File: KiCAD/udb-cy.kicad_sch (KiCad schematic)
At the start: 15 parts, among them J0 USB_C_Receptacle, J1 JST-SH-04, J2 JST-SUR-04, J3 Conn_01x04

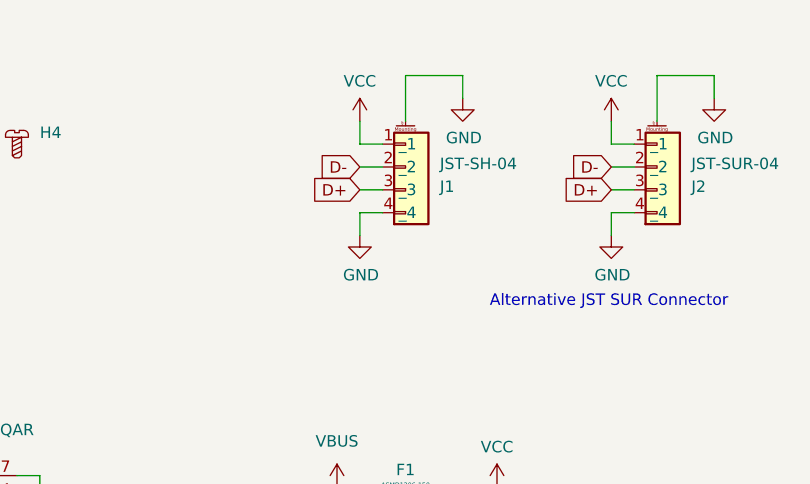
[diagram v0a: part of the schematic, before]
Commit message: update-2025-11-20
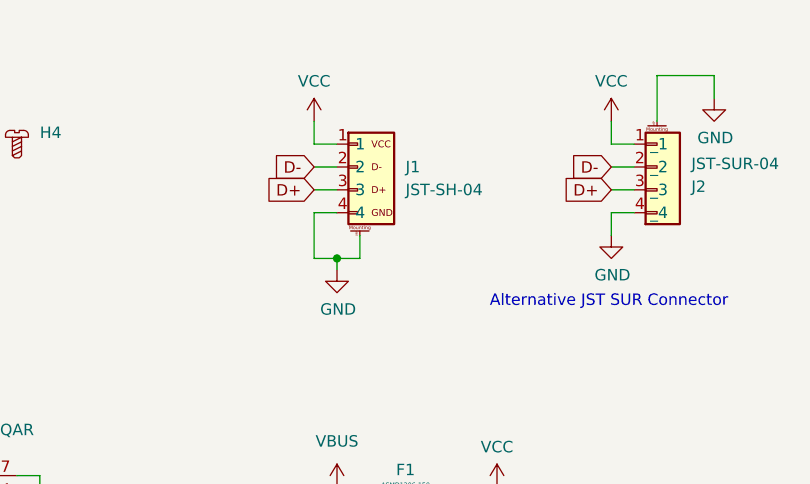
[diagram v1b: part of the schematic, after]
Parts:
- J1: symbol ts-kicad-lib:CONN_04 -> ts-keyboard-lib:CONN_UDB
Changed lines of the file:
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@@
+	)
+	(junction
+		(at 144.78 48.26)
+		(diameter 0)
+		(color 0 0 0 0)
 	)
 	(junction
@@
 	(wire
 		(pts
-			(xy 147.32 45.72) (xy 147.32 43.18)
+			(xy 144.78 49.53) (xy 144.78 48.26)
 		)
 		(stroke
@@
 	(wire
 		(pts
-			(xy 152.4 27.94) (xy 152.4 33.02)
-		)
-		(stroke
-			(width 0)
-			(type default)
-		)
-	)
-	(wire
-		(pts
 			(xy 38.1 78.74) (xy 38.1 83.82)
 		)
@@
 	(wire
 		(pts
+			(xy 144.78 48.26) (xy 142.24 48.26)
+		)
+		(stroke
+			(width 0)
+			(type default)
+		)
+	)
+	(wire
+		(pts
 			(xy 144.78 76.2) (xy 148.59 76.2)
 		)
@@
 	(wire
 		(pts
-			(xy 147.32 40.64) (xy 149.86 40.64)
-		)
-		(stroke
-			(width 0)
-			(type default)
-		)
-	)
-	(wire
-		(pts
 			(xy 156.21 76.2) (xy 160.02 76.2)
 		)
@@
 	(wire
 		(pts
+			(xy 147.32 45.72) (xy 147.32 48.26)
+		)
+		(stroke
+			(width 0)
+			(type default)
+		)
+	)
+	(wire
+		(pts
 			(xy 45.72 43.18) (xy 50.8 43.18)
 		)
@@
 	(wire
 		(pts
+			(xy 142.24 43.18) (xy 144.78 43.18)
+		)
+		(stroke
+			(width 0)
+			(type default)
+		)
+	)
+	(wire
+		(pts
 			(xy 180.34 27.94) (xy 180.34 33.02)
 		)
@@
 	(wire
 		(pts
+			(xy 144.78 48.26) (xy 147.32 48.26)
+		)
+		(stroke
+			(width 0)
+			(type default)
+		)
+	)
+	(wire
+		(pts
 			(xy 66.04 45.72) (xy 50.8 45.72)
 		)
@@
 	(wire
 		(pts
-			(xy 158.75 27.94) (xy 152.4 27.94)
-		)
-		(stroke
-			(width 0)
-			(type default)
-		)
-	)
-	(wire
-		(pts
-			(xy 147.32 33.02) (xy 147.32 35.56)
+			(xy 142.24 33.02) (xy 142.24 35.56)
 		)
 		(stroke
@@
 	(wire
 		(pts
+			(xy 142.24 38.1) (xy 144.78 38.1)
+		)
+		(stroke
+			(width 0)
+			(type default)
+		)
+	)
+	(wire
+		(pts
 			(xy 48.26 86.36) (xy 50.8 86.36)
 		)
@@
 	(wire
 		(pts
+			(xy 142.24 48.26) (xy 142.24 43.18)
+		)
+		(stroke
+			(width 0)
+			(type default)
+		)
+	)
+	(wire
+		(pts
 			(xy 109.22 80.01) (xy 111.76 80.01)
 		)
@@
 	(wire
 		(pts
-			(xy 158.75 30.48) (xy 158.75 27.94)
-		)
-		(stroke
-			(width 0)
-			(type default)
-		)
-	)
-	(wire
-		(pts
-			(xy 147.32 35.56) (xy 149.86 35.56)
-		)
-		(stroke
-			(width 0)
-			(type default)
-		)
-	)
-	(wire
-		(pts
 			(xy 48.26 30.48) (xy 50.8 30.48)
 		)
@@
 	(wire
 		(pts
+			(xy 142.24 35.56) (xy 144.78 35.56)
+		)
+		(stroke
+			(width 0)
+			(type default)
+		)
+	)
+	(wire
+		(pts
 			(xy 40.64 78.74) (xy 38.1 78.74)
 		)
@@
 	(wire
 		(pts
-			(xy 147.32 43.18) (xy 149.86 43.18)
-		)
-		(stroke
-			(width 0)
-			(type default)
-		)
-	)
-	(wire
-		(pts
-			(xy 149.86 38.1) (xy 147.32 38.1)
+			(xy 142.24 40.64) (xy 144.78 40.64)
 		)
 		(stroke
@@
 	(global_label "D+"
 		(shape input)
-		(at 147.32 40.64 180)
+		(at 142.24 40.64 180)
 		(effects
 			(font
@@
 		)
 		(property "Intersheetrefs" "${INTERSHEET_REFS}"
-			(at 147.32 40.64 0)
+			(at 142.24 40.64 0)
 			(effects
 				(font
@@
 	(global_label "D-"
 		(shape input)
-		(at 147.32 38.1 180)
+		(at 142.24 38.1 180)
 		(effects
 			(font
@@
 		)
 		(property "Intersheetrefs" "${INTERSHEET_REFS}"
-			(at 147.32 38.1 0)
+			(at 142.24 38.1 0)
 			(effects
 				(font
@@
 	(symbol
 		(lib_id "power:GND")
-		(at 147.32 45.72 0)
+		(at 144.78 49.53 0)
 		(unit 1)
 		(exclude_from_sim no)
@@
 		(dnp no)
 		(property "Reference" "#PWR0104"
-			(at 147.32 52.07 0)
+			(at 144.78 55.88 0)
 			(effects
 				(font
@@
 		)
 		(property "Value" "GND"
-			(at 147.447 50.1142 0)
+			(at 144.907 53.9242 0)
 			(effects
 				(font
@@
 		)
 		(property "Footprint" ""
-			(at 147.32 45.72 0)
+			(at 144.78 49.53 0)
 			(effects
 				(font
@@
 		)
 		(property "Datasheet" ""
-			(at 147.32 45.72 0)
+			(at 144.78 49.53 0)
 			(effects
 				(font
@@
 		)
 		(property "Description" ""
-			(at 147.32 45.72 0)
+			(at 144.78 49.53 0)
 			(effects
 				(font
@@
 	(symbol
 		(lib_id "power:VCC")
-		(at 147.32 33.02 0)
+		(at 142.24 33.02 0)
 		(unit 1)
 		(exclude_from_sim no)
@@
 		(dnp no)
 		(property "Reference" "#PWR0103"
-			(at 147.32 36.83 0)
+			(at 142.24 36.83 0)
 			(effects
 				(font
@@
 		)
 		(property "Value" "VCC"
-			(at 147.32 28.575 0)
+			(at 142.24 28.575 0)
 			(effects
 				(font
@@
 		)
 		(property "Footprint" ""
-			(at 147.32 33.02 0)
+			(at 142.24 33.02 0)
 			(effects
 				(font
@@
 		)
 		(property "Datasheet" ""
-			(at 147.32 33.02 0)
+			(at 142.24 33.02 0)
 			(effects
 				(font
@@
 		)
 		(property "Description" ""
-			(at 147.32 33.02 0)
+			(at 142.24 33.02 0)
 			(effects
 				(font
@@
 	)
 	(symbol
-		(lib_id "ts-kicad-lib:CONN_04")
-		(at 152.4 38.1 0)
-		(mirror x)
+		(lib_id "ts-keyboard-lib:CONN_UDB")
+		(at 147.32 40.64 0)
 		(unit 1)
 		(exclude_from_sim no)
@@
 		(dnp no)
 		(property "Reference" "J1"
-			(at 156.21 40.2845 0)
+			(at 152.4 38.1 0)
 			(effects
 				(font
@@
 		)
 		(property "Value" "JST-SH-04"
-			(at 156.21 37.7445 0)
+			(at 152.4 40.64 0)
 			(effects
 				(font
@@
 		)
 		(property "Footprint" "Connector_JST:JST_SH_SM04B-SRSS-TB_1x04-1MP_P1.00mm_Horizontal"
-			(at 152.4 38.1 0)
-			(effects
-				(font
-					(size 1.27 1.27)
-				)
-				(hide yes)
-			)
-		)
-		(property "Datasheet" ""
-			(at 152.4 38.1 0)
-			(effects
-				(font
-					(size 1.27 1.27)
-				)
-				(hide yes)
-			)
-		)
-		(property "Description" ""
-			(at 152.4 38.1 0)
+			(at 147.32 27.94 0)
+			(effects
+				(font
+					(size 1.27 1.27)
+				)
+				(hide yes)
+			)
+		)
+		(property "Datasheet" "https://unified-daughterboard.github.io"
+			(at 147.32 30.48 0)
+			(effects
+				(font
+					(size 1.27 1.27)
+				)
+				(hide yes)
+			)
+		)
+		(property "Description" "Unified Daughterboard C Series"
+			(at 147.32 25.4 0)
 			(effects
 				(font
@@
 					(unit 1)
 				)
-			)
-		)
-	)
-	(symbol
-		(lib_id "power:GND")
-		(at 158.75 30.48 0)
-		(unit 1)
-		(exclude_from_sim no)
-		(in_bom yes)
-		(on_board yes)
-		(dnp no)
-		(property "Reference" "#PWR013"
-			(at 158.75 36.83 0)
-			(effects
-				(font
-					(size 1.27 1.27)
-				)
-				(hide yes)
-			)
-		)
-		(property "Value" "GND"
-			(at 158.877 34.8742 0)
-			(effects
-				(font
-					(size 1.27 1.27)
-				)
-			)
-		)
-		(property "Footprint" ""
-			(at 158.75 30.48 0)
-			(effects
-				(font
-					(size 1.27 1.27)
-				)
-				(hide yes)
-			)
-		)
-		(property "Datasheet" ""
-			(at 158.75 30.48 0)
-			(effects
-				(font
-					(size 1.27 1.27)
-				)
-				(hide yes)
-			)
-		)
-		(property "Description" ""
-			(at 158.75 30.48 0)
-			(effects
-				(font
-					(size 1.27 1.27)
-				)
-			)
-		)
-		(pin "1"
-		)
-		(instances
-			(project "udb-cy"
-				(path "/45b81b3f-a376-44a8-a955-c3164d7947b8"
-					(reference "#PWR013")
-					(unit 1)
-				)

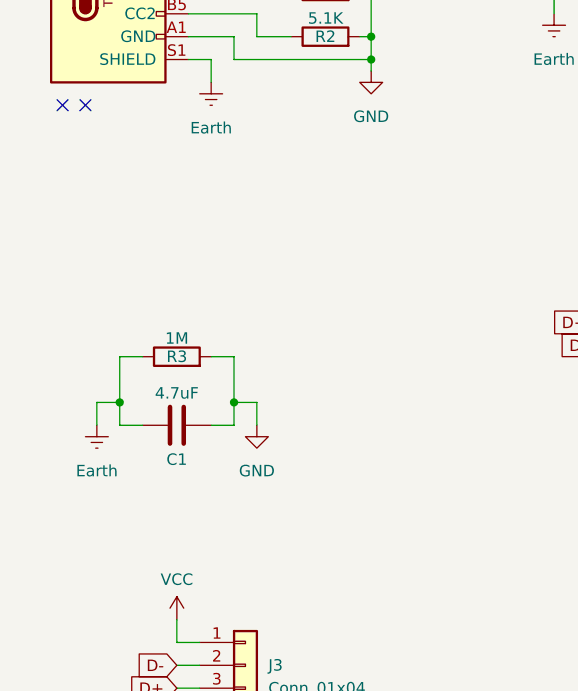
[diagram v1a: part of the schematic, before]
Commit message: .
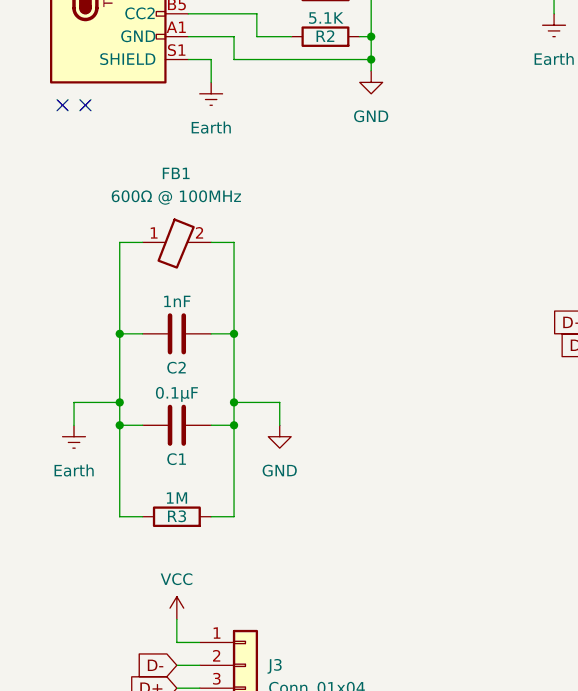
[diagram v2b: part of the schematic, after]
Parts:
- added C2: 1nF, Capacitor_SMD:C_0603_1608Metric, symbol Device:C
- added FB1: 600Ω @ 100MHz, Inductor_SMD:L_0603_1608Metric, symbol ts-kicad-lib:Ferrite_Bead
- C1: value 4.7uF -> 0.1µF
- H1, H2, H3, H4: value ~ -> (none)
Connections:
- net Earth: now also C2.1, FB1.1
- net GND: now also C2.2, FB1.2
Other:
- moved on the sheet: R3

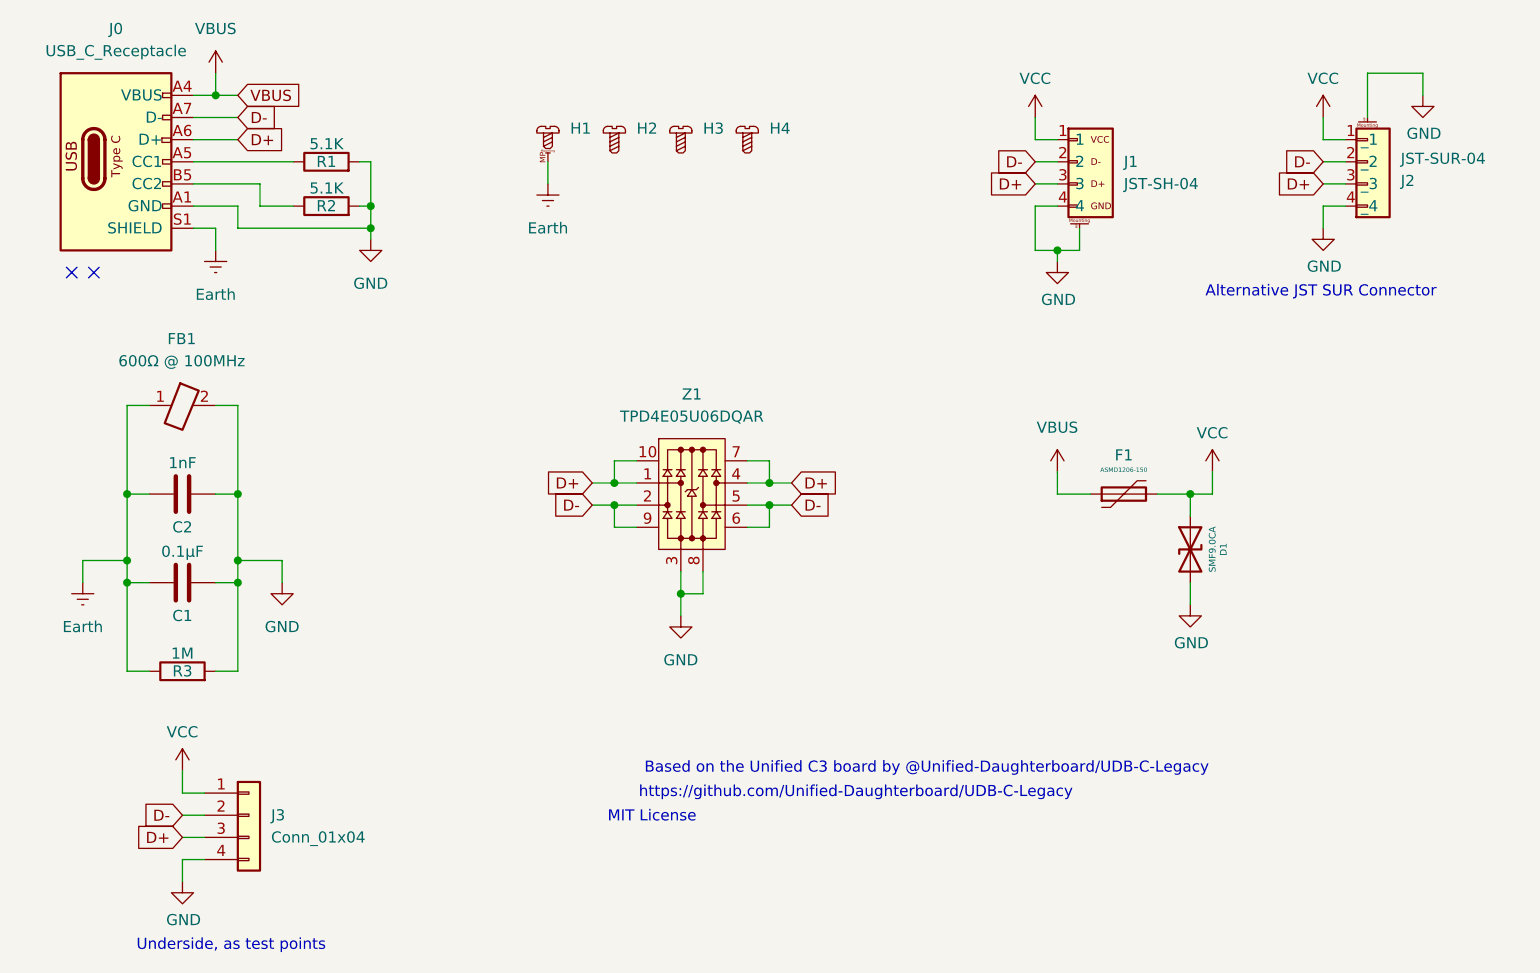
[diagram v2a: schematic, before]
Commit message: updated
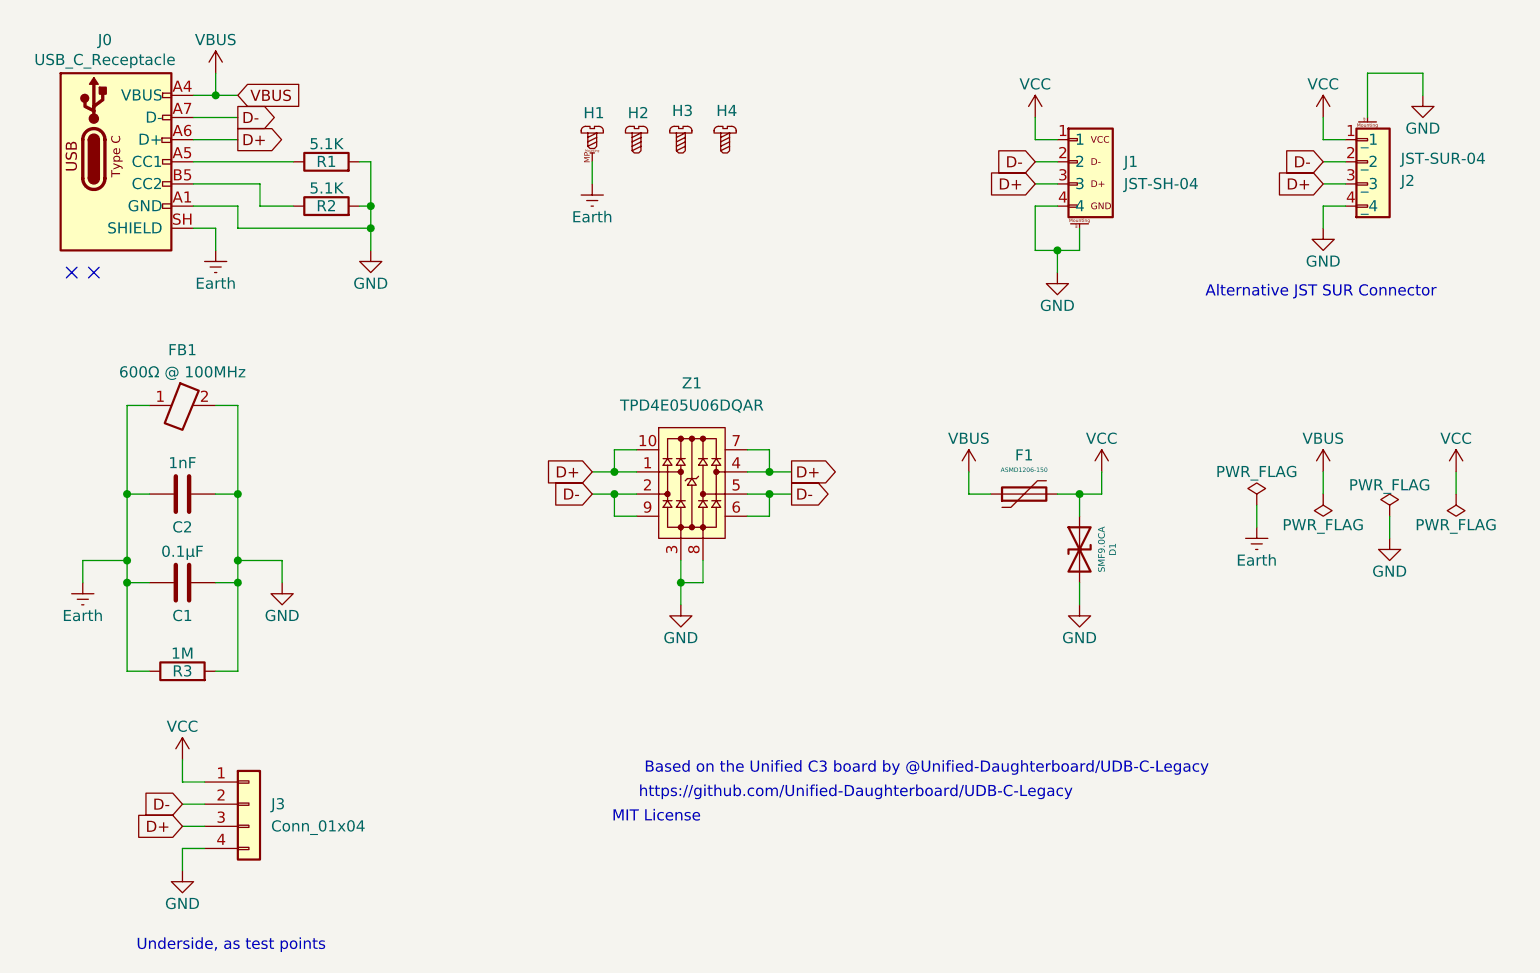
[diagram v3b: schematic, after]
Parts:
- J1: footprint Connector_JST:JST_SH_SM04B-SRSS-TB_1x04-1MP_P1.00mm_Horizontal -> ts-keyboard-lib:JST_SH_SM04B-SRSS-TB_1x04-1MP_P1.00mm_Horizontal
- R1, R2, R3: footprint Resistors_SMD:R_0603 -> Resistor_SMD:R_0603_1608Metric_Pad0.98x0.95mm_HandSolder
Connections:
- net Earth: now also J0.SH (SHIELD); no longer J0.S1 (SHIELD)
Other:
- moved on the sheet: D1, F1, H1, H2, H4, J3, Z1
